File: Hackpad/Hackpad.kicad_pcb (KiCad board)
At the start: 2 copper layers, 42 x 61 mm, 8 parts, among them SW1 SW_Push_45deg, SW2 SW_Push_45deg, SW3 SW_Push_45deg, SW4 SW_Push_45deg, SW5 RotaryEncoder_Switch_MP, U1 XIAO-RP2040-DIP

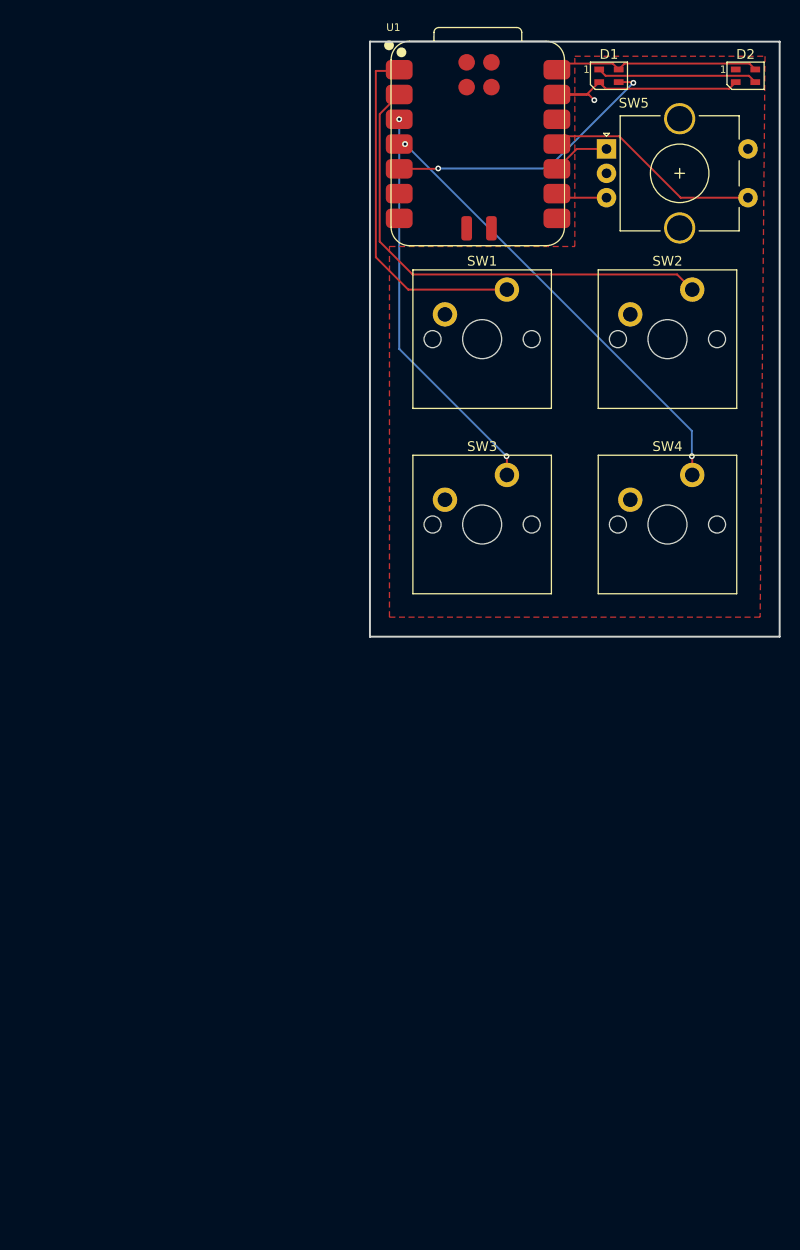
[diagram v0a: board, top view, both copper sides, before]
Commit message: Resubmission
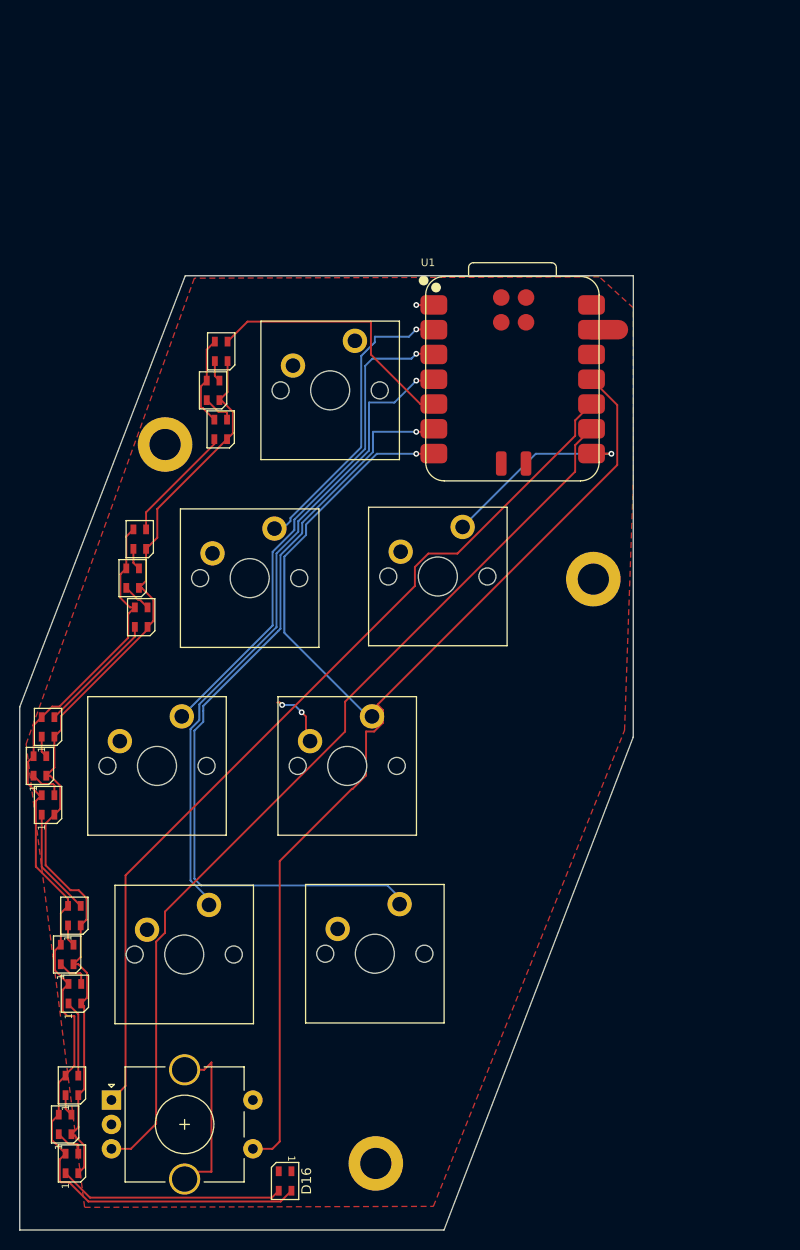
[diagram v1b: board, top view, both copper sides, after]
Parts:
- added D10: SK6805, LED_SMD:LED_SK6805_PLCC4_2.4x2.7mm_P1.3mm, F.Cu at (52.7, 114.6)
- added D11: SK6805, LED_SMD:LED_SK6805_PLCC4_2.4x2.7mm_P1.3mm, F.Cu at (52.0, 118.6)
- added D12: SK6805, LED_SMD:LED_SK6805_PLCC4_2.4x2.7mm_P1.3mm, F.Cu at (52.8, 122.6)
- added D13: SK6805, LED_SMD:LED_SK6805_PLCC4_2.4x2.7mm_P1.3mm, F.Cu at (52.5, 132.0)
- added D14: SK6805, LED_SMD:LED_SK6805_PLCC4_2.4x2.7mm_P1.3mm, F.Cu at (51.8, 136.0)
- added D15: SK6805, LED_SMD:LED_SK6805_PLCC4_2.4x2.7mm_P1.3mm, F.Cu at (52.5, 140.0)
- added D16: SK6805, LED_SMD:LED_SK6805_PLCC4_2.4x2.7mm_P1.3mm, F.Cu at (74.3, 141.8)
- added D3: SK6805, LED_SMD:LED_SK6805_PLCC4_2.4x2.7mm_P1.3mm, F.Cu at (67.7, 64.8)
- added D4: SK6805, LED_SMD:LED_SK6805_PLCC4_2.4x2.7mm_P1.3mm, F.Cu at (59.4, 76.0)
- added D5: SK6805, LED_SMD:LED_SK6805_PLCC4_2.4x2.7mm_P1.3mm, F.Cu at (58.7, 80.0)
- added D6: SK6805, LED_SMD:LED_SK6805_PLCC4_2.4x2.7mm_P1.3mm, F.Cu at (59.5, 84.0)
- added D7: SK6805, LED_SMD:LED_SK6805_PLCC4_2.4x2.7mm_P1.3mm, F.Cu at (50.0, 95.2)
- added D8: SK6805, LED_SMD:LED_SK6805_PLCC4_2.4x2.7mm_P1.3mm, F.Cu at (49.2, 99.2)
- added D9: SK6805, LED_SMD:LED_SK6805_PLCC4_2.4x2.7mm_P1.3mm, F.Cu at (50.0, 103.2)
- added REF**: MountingHole_3.2mm_M3_DIN965_Pad, MountingHole:MountingHole_3.2mm_M3_DIN965_Pad, F.Cu at (62.0, 66.3)
- added REF**: MountingHole_3.2mm_M3_DIN965_Pad, MountingHole:MountingHole_3.2mm_M3_DIN965_Pad, F.Cu at (105.9, 80.1)
- added REF**: MountingHole_3.2mm_M3_DIN965_Pad, MountingHole:MountingHole_3.2mm_M3_DIN965_Pad, F.Cu at (83.6, 140.0)
- added SW6: SW_Push_45deg, PCM_Switch_Keyboard_Cherry_MX:SW_Cherry_MX_PCB_1.00u, F.Cu at (83.5, 118.5)
- added SW7: SW_Push_45deg, PCM_Switch_Keyboard_Cherry_MX:SW_Cherry_MX_PCB_1.00u, F.Cu at (80.7, 99.2)
- added SW8: SW_Push_45deg, PCM_Switch_Keyboard_Cherry_MX:SW_Cherry_MX_PCB_1.00u, F.Cu at (90.0, 79.8)
- moved SW5 109.9 mm to (56.5, 133.5)
- moved SW4 66.3 mm to (64.0, 118.6)
- moved D2 63.4 mm to (66.9, 60.8), turned to 90 degrees
- moved SW2 49.3 mm to (70.7, 80.0)
- moved D1 48.8 mm to (67.8, 56.8), turned to 90 degrees
- moved SW3 41.5 mm to (61.2, 99.2)
- moved U1 24.4 mm to (97.5, 59.6)
- moved SW1 16.4 mm to (78.9, 60.8)
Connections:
- D2 pad 1: unconnected-(D2-DOUT-Pad1) -> Net-(D2-DOUT)
- U1 pad 6: unconnected-(U1-GPIO7/SCL-Pad6) -> Net-(U1-GPIO7/SCL)
- U1 pad 7: unconnected-(U1-GPIO0/TX-Pad7) -> Net-(U1-GPIO0/TX)
- U1 pad 8: unconnected-(U1-GPIO1/RX-Pad8) -> Net-(U1-GPIO1/RX)
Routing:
- net +5V: track 21.3 -> 114.2 mm
- net Net-(U1-GPIO2/SCK): track 5.26 -> 95.4 mm
- net Net-(U1-GPIO4/MISO): track 5.93 -> 93.5 mm
- net GND: track 23.5 -> 109.3 mm, vias 1 -> 2
- net Net-(U1-GPIO7/SCL): track 0.00 -> 81.5 mm, vias 0 -> 1
- net Net-(U1-GPIO3/MOSI): track 22.5 -> 97.6 mm
- net Net-(U1-GPIO0/TX): track 0.00 -> 40.2 mm, vias 0 -> 1
- net Net-(U1-GPIO26/ADC0/A0): track 36.4 -> 1.80 mm, vias 0 -> 1
- net Net-(D15-DOUT): track 0.00 -> 23.2 mm
- net Net-(U1-GPIO29/ADC3/A3): track 46.1 -> 67.3 mm, vias 2 -> 1
- net Net-(U1-GPIO1/RX): track 0.00 -> 20.4 mm, vias 0 -> 1
- net Net-(U1-GPIO27/ADC1/A1): track 50.0 -> 30.8 mm, vias 0 -> 1
- net unconnected-(SW5-PadMP): track 0.00 -> 17.3 mm
- net Net-(D1-DOUT): track 16.5 -> 2.19 mm
- net Net-(D6-DOUT): track 0.00 -> 12.7 mm
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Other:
- board size 42 x 61 mm -> 62.9 x 97.8 mm
